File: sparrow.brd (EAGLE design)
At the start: 80 x 80 mm, 196 parts, among them IC1 LAN8720AVIAS, IC2 TLV320AIC3100VIAS, IC3 TPS2500, IC4 SKYWORKS_AAT4280ASC70JW-8-NOT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, IC5 SKYWORKS_AAT4280ASC70JW-8-NOT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, IC6 SKYWORKS_AAT4280ASC70JW-8-NOT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, IC7 SKYWORKS_AAT4280ASC70JW-8-NOT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, IC8 SKYWORKS_AAT4280ASC70JW-8-NOT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, IC9 FXMA10820-DFN, X1 ABS07-32768, X2 12MHz, X3 32768, X4 50MHZ, X5 16MHz

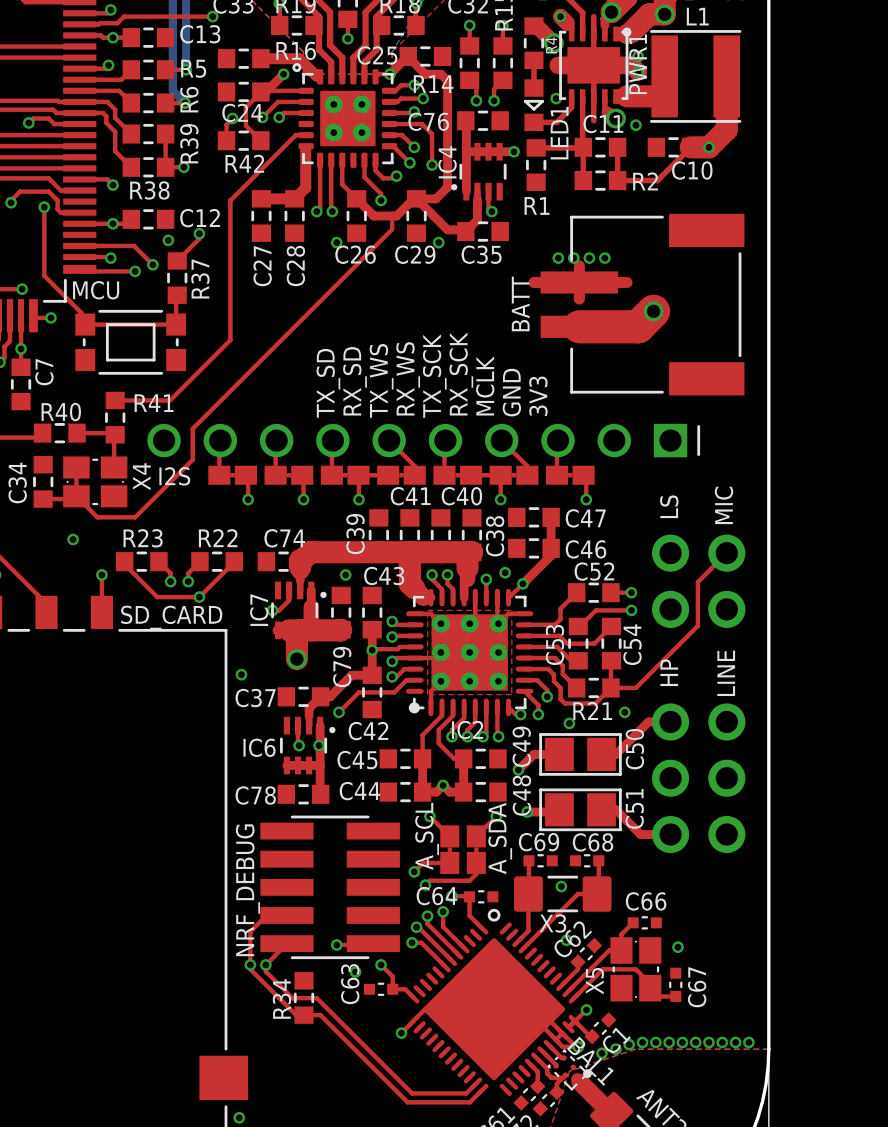
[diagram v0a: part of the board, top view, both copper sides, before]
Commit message: RC1
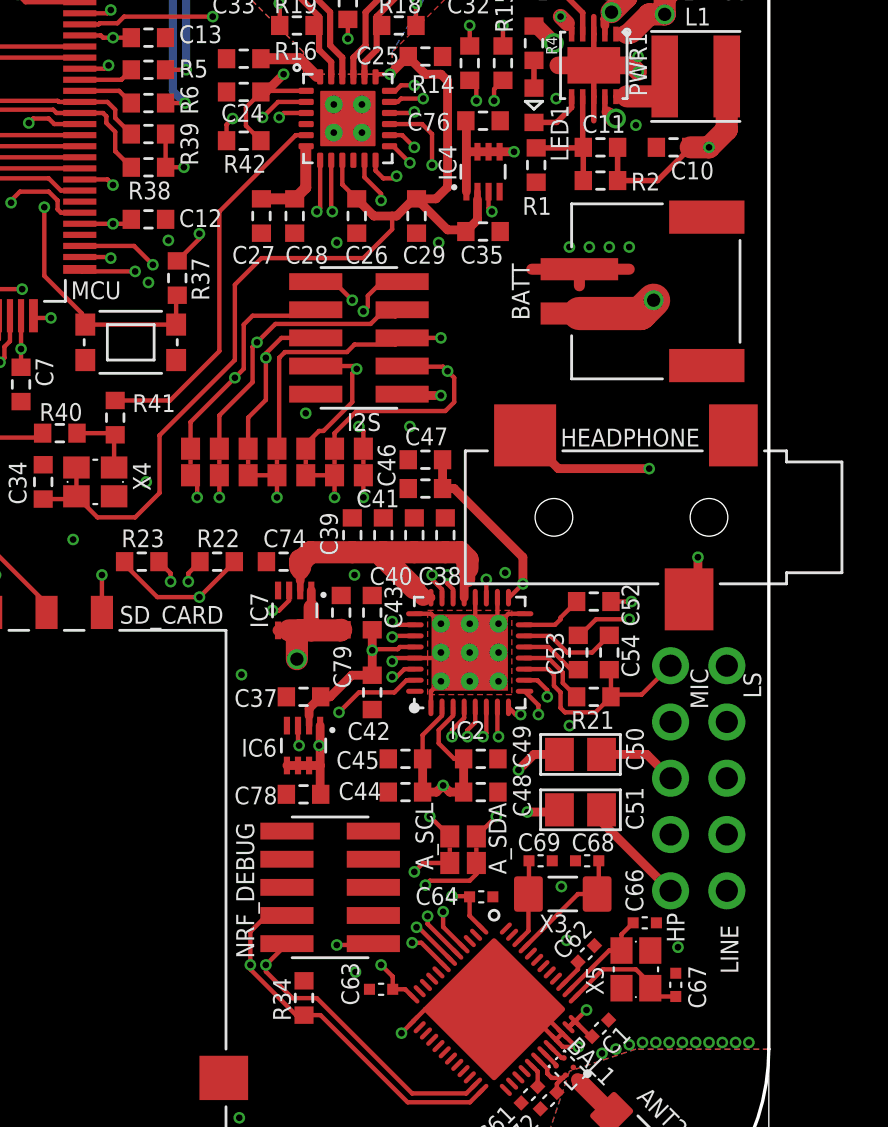
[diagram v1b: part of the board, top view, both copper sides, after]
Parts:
- added HEADPHONE: AUDIOJACK-STEREO-3PCUI_SJ_3523, anykey:CUI_SJ_3523_SMT
- I2S: value HEADER-1X10ROUND -> HEADER-2X5SMD-1.27MM; device anykey:1X10_ROUND -> anykey:2X05_SMT
- moved MCLK 9.36 mm to (61.7, 36.5), turned to 270 degrees
- moved RX_SCK 8.12 mm to (60.4, 36.5), turned to 270 degrees
- moved TX_SCK 6.89 mm to (59.1, 36.5), turned to 270 degrees
- moved LS 5.68 mm to (78.1, 26.0)
- moved MIC 5.68 mm to (75.6, 26.0)
- moved RX_WS 5.65 mm to (57.8, 36.5), turned to 270 degrees
- moved C46 5.59 mm to (64.5, 35.3)
- moved C47 5.55 mm to (64.5, 36.6)
- moved I2S 5.33 mm to (61.5, 42.1), turned to 90 degrees
- moved TX_WS 4.42 mm to (56.5, 36.5), turned to 270 degrees
- moved RX_SD 3.20 mm to (55.2, 36.5), turned to 270 degrees
- moved HP 2.54 mm to (75.6, 19.7)
- moved LINE 2.54 mm to (78.1, 19.7)
- moved TX_SD 1.99 mm to (53.9, 36.5), turned to 270 degrees
- moved C40 1.20 mm to (64.0, 33.2)
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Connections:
- net MIC renamed N$4
- net GND: now also HEADPHONE.1
- net HP_L: now also HEADPHONE.2
- net HP_R: now also HEADPHONE.3
- net I2S_RX_MCLK: now also I2S.9; no longer I2S.3
- net I2S_RX_SCK: now also I2S.3; no longer I2S.4
- net I2S_RX_SD: now also I2S.7; no longer I2S.8
- net I2S_RX_WS: now also I2S.5; no longer I2S.6
- net I2S_TX_SCK: now also I2S.4; no longer I2S.5
- net I2S_TX_SD: now also I2S.8; no longer I2S.9
- net I2S_TX_WS: now also I2S.6; no longer I2S.7
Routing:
- net HP_L: track 3.72 -> 24.7 mm, vias 0 -> 1
- net HP_R: track 3.58 -> 22.6 mm, vias 0 -> 1
- net I2S_RX_WS: track 20.0 -> 31.7 mm, vias 1 -> 2
- net I2S_TX_MCLK: track 39.8 -> 51.0 mm, vias 1 -> 2
- net I2S_RX_SD: track 22.1 -> 30.5 mm, vias 1 -> 2
- net I2S_TX_SD: track 35.9 -> 43.6 mm, vias 1 -> 2
- net I2S_RX_SCK: track 24.8 -> 32.2 mm, vias 1 -> 2
- net SPKM: track 15.6 -> 21.6 mm
- net AUDIO_MCLK: track 25.1 -> 19.2 mm
- net VD33: track 595.4 -> 601.2 mm, vias 32 -> 33
- net N$4: track 15.4 -> 10.2 mm
- net SPKP: track 19.3 -> 24.3 mm
- net I2S_RX_MCLK: track 34.4 -> 30.0 mm, vias 1 -> 3
- net VAUDIO33: track 47.3 -> 51.2 mm
- net LINEIN1: track 8.54 -> 11.8 mm
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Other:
- board text removed: "TX_SD RX_SD TX_WS RX_WS TX_SCK RX_SCK MCLK GND 3V3"
